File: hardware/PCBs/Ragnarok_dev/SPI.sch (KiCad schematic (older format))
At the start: 5 parts, among them U7 AB0815, U8 BMP388

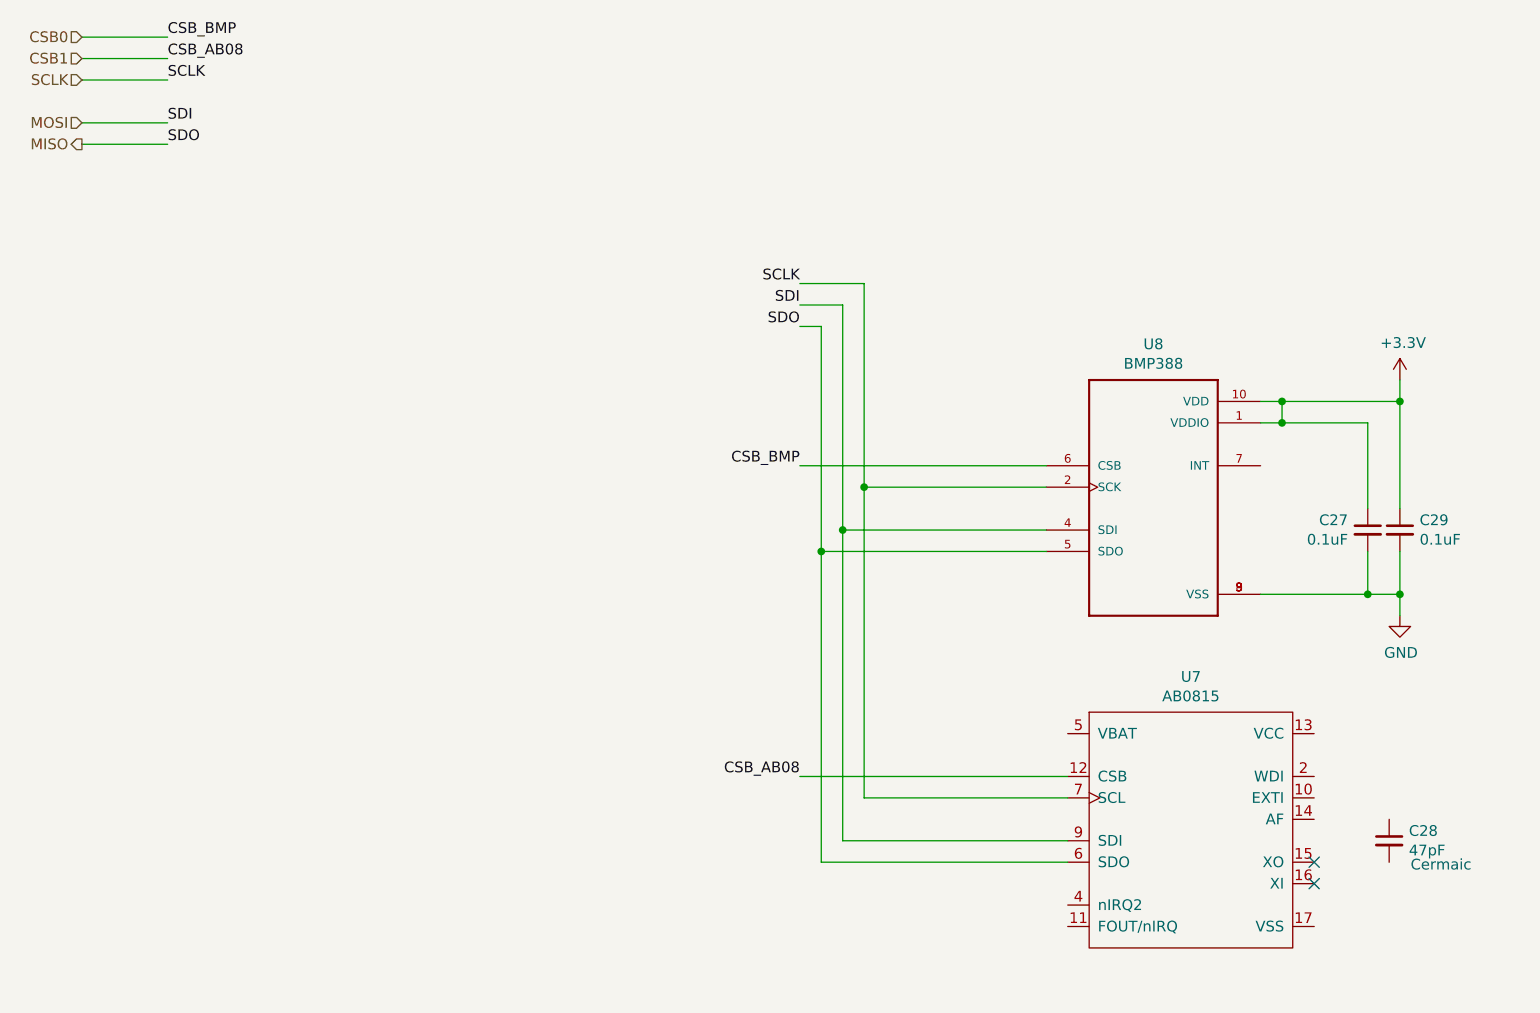
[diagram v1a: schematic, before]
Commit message: update
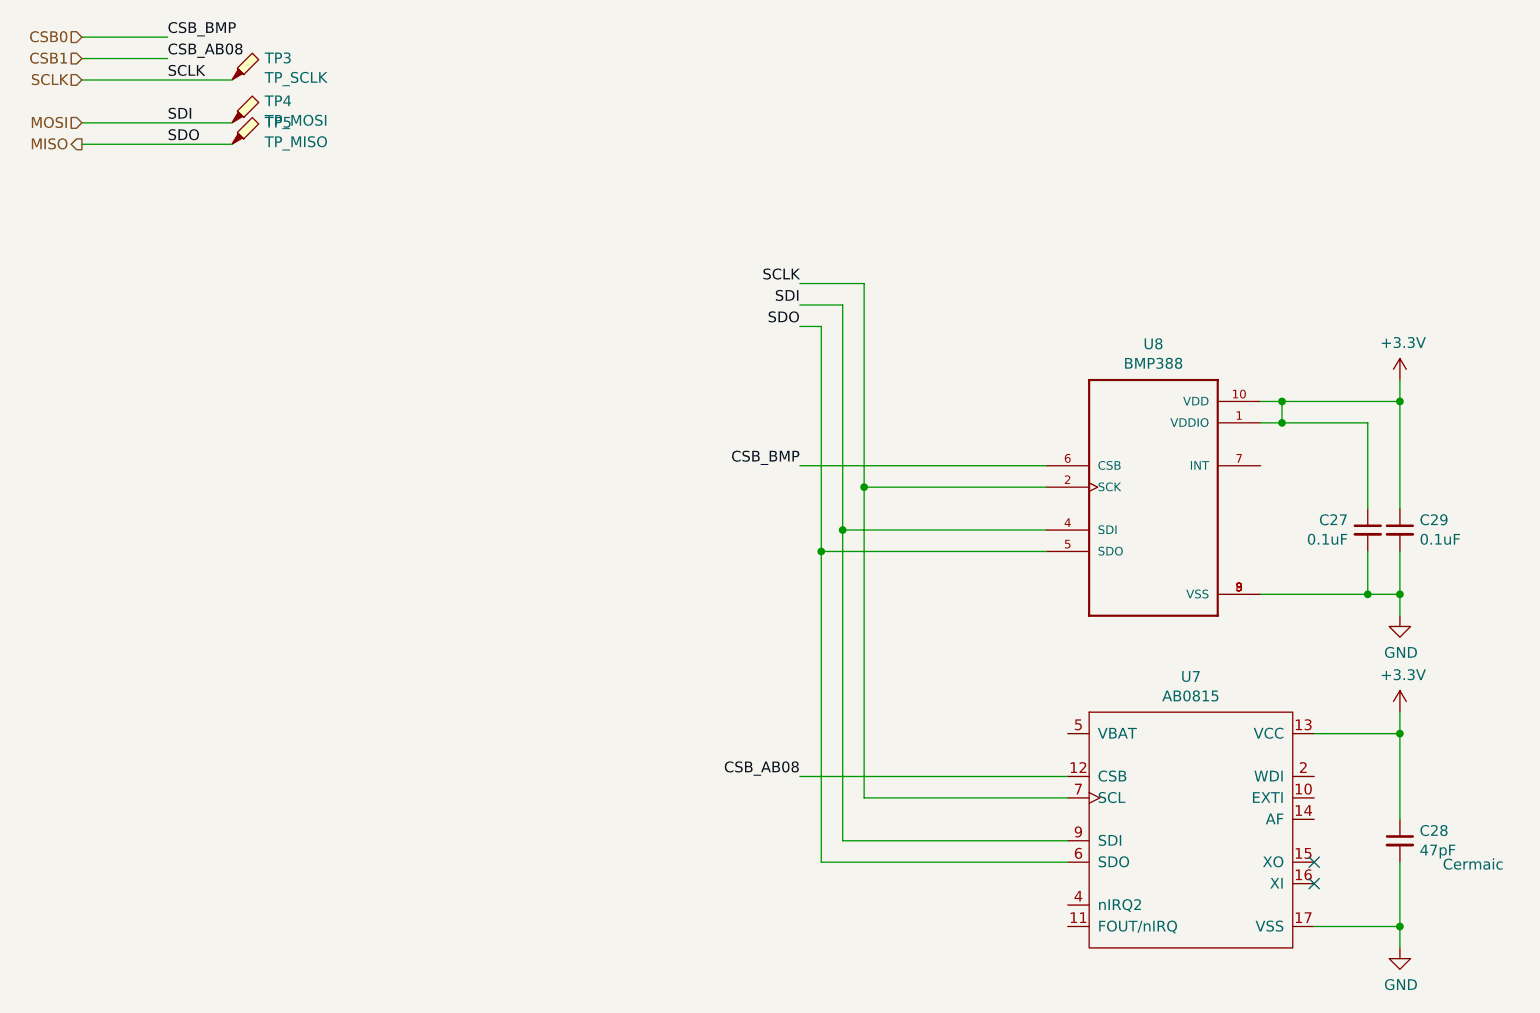
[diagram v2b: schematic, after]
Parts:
- added TP3: TP_SCLK, TestPoint:TestPoint_Pad_1.0x1.0mm, symbol Connector:TestPoint_Probe
- added TP4: TP_MOSI, TestPoint:TestPoint_Pad_1.0x1.0mm, symbol Connector:TestPoint_Probe
- added TP5: TP_MISO, TestPoint:TestPoint_Pad_1.0x1.0mm, symbol Connector:TestPoint_Probe
- C27, C28, C29: footprint (none) -> Capacitor_SMD:C_0603_1608Metric_Pad1.05x0.95mm_HandSolder
- U7: footprint (none) -> Package_DFN_QFN:QFN-16-1EP_5x5mm_P0.8mm_EP2.7x2.7mm
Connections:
- net +3V3: now also C28.1, U7.13 (VCC)
- net GND: now also C28.2, U7.17 (VSS)
- net MISO: now also TP5.1
- net MOSI: now also TP4.1
- net SCLK: now also TP3.1
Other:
- moved on the sheet: C28
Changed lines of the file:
@@
 F 0 "C29" H 7592 3446 50  0000 L CNN
 F 1 "0.1uF" H 7592 3355 50  0000 L CNN
-F 2 "" H 7500 3400 50  0001 C CNN
+F 2 "Capacitor_SMD:C_0603_1608Metric_Pad1.05x0.95mm_HandSolder" H 7500 3400 50  0001 C CNN
 F 3 "~" H 7500 3400 50  0001 C CNN
 	1    7500 3400
@@
 F 0 "U7" H 6525 4715 50  0000 C CNN
 F 1 "AB0815" H 6525 4624 50  0000 C CNN
-F 2 "" H 6550 4600 50  0001 C CNN
+F 2 "Package_DFN_QFN:QFN-16-1EP_5x5mm_P0.8mm_EP2.7x2.7mm" H 6550 4600 50  0001 C CNN
 F 3 "" H 6550 4600 50  0001 C CNN
 	1    5650 4400
@@
 L Device:C_Small C28
 U 1 1 5E1BCE97
-P 7450 4850
-F 0 "C28" H 7542 4896 50  0000 L CNN
-F 1 "47pF" H 7542 4805 50  0000 L CNN
-F 2 "" H 7450 4850 50  0001 C CNN
-F 3 "~" H 7450 4850 50  0001 C CNN
-	1    7450 4850
-	1    0    0    -1
-$EndComp
-Text Notes 7550 5000 0    50   ~ 0
+P 7500 4850
+F 0 "C28" H 7592 4896 50  0000 L CNN
+F 1 "47pF" H 7592 4805 50  0000 L CNN
+F 2 "Capacitor_SMD:C_0603_1608Metric_Pad1.05x0.95mm_HandSolder" H 7500 4850 50  0001 C CNN
+F 3 "~" H 7500 4850 50  0001 C CNN
+	1    7500 4850
+	1    0    0    -1
+$EndComp
+Text Notes 7700 5000 0    50   ~ 0
 Cermaic\n
 $Comp
@@
 F 0 "C27" H 7442 3446 50  0000 L CNN
 F 1 "0.1uF" H 7442 3355 50  0000 L CNN
-F 2 "" H 7350 3400 50  0001 C CNN
+F 2 "Capacitor_SMD:C_0603_1608Metric_Pad1.05x0.95mm_HandSolder" H 7350 3400 50  0001 C CNN
 F 3 "~" H 7350 3400 50  0001 C CNN
 	1    7350 3400
@@
 Text Label 1750 1600 0    50   ~ 0
 SDO
-Wire Wire Line
-	1350 1300 1750 1300
-Wire Wire Line
-	1350 1500 1750 1500
-Wire Wire Line
-	1350 1600 1750 1600
 Text HLabel 1350 1100 0    50   Input ~ 0
 CSB0
@@
 NoConn ~ 7100 4950
 NoConn ~ 7100 5050
+$Comp
+L Connector:TestPoint_Probe TP?
+U 1 1 5E857A15
+P 2050 1300
+AR Path="/5E857A15" Ref="TP?"  Part="1"
+AR Path="/5E1A0CB7/5E857A15" Ref="TP3"  Part="1"
+F 0 "TP3" H 2203 1401 50  0000 L CNN
+F 1 "TP_SCLK" H 2203 1310 50  0000 L CNN
+F 2 "TestPoint:TestPoint_Pad_1.0x1.0mm" H 2250 1300 50  0001 C CNN
+F 3 "~" H 2250 1300 50  0001 C CNN
+	1    2050 1300
+	1    0    0    -1
+$EndComp
+$Comp
+L Connector:TestPoint_Probe TP?
+U 1 1 5E857A1B
+P 2050 1600
+AR Path="/5E857A1B" Ref="TP?"  Part="1"
+AR Path="/5E1A0CB7/5E857A1B" Ref="TP5"  Part="1"
+F 0 "TP5" H 2203 1701 50  0000 L CNN
+F 1 "TP_MISO" H 2203 1610 50  0000 L CNN
+F 2 "TestPoint:TestPoint_Pad_1.0x1.0mm" H 2250 1600 50  0001 C CNN
+F 3 "~" H 2250 1600 50  0001 C CNN
+	1    2050 1600
+	1    0    0    -1
+$EndComp
+$Comp
+L Connector:TestPoint_Probe TP?
+U 1 1 5E857A21
+P 2050 1500
+AR Path="/5E857A21" Ref="TP?"  Part="1"
+AR Path="/5E1A0CB7/5E857A21" Ref="TP4"  Part="1"
+F 0 "TP4" H 2203 1601 50  0000 L CNN
+F 1 "TP_MOSI" H 2203 1510 50  0000 L CNN
+F 2 "TestPoint:TestPoint_Pad_1.0x1.0mm" H 2250 1500 50  0001 C CNN
+F 3 "~" H 2250 1500 50  0001 C CNN
+	1    2050 1500
+	1    0    0    -1
+$EndComp
+Wire Wire Line
+	1350 1500 2050 1500
+Wire Wire Line
+	1350 1600 2050 1600
+Wire Wire Line
+	1350 1300 2050 1300
+$Comp
+L power:+3.3V #PWR0165
+U 1 1 5E85DA72
+P 7500 4250
+F 0 "#PWR0165" H 7500 4100 50  0001 C CNN
+F 1 "+3.3V" H 7515 4423 50  0000 C CNN
+F 2 "" H 7500 4250 50  0001 C CNN
+F 3 "" H 7500 4250 50  0001 C CNN
+	1    7500 4250
+	1    0    0    -1
+$EndComp
+Wire Wire Line
+	7500 4250 7500 4350
+Wire Wire Line
+	7500 4350 7100 4350
+Wire Wire Line
+	7500 4350 7500 4750
+Connection ~ 7500 4350
+Wire Wire Line
+	7500 4950 7500 5250
+Wire Wire Line
+	7500 5250 7100 5250
+$Comp
+L power:GND #PWR0166
+U 1 1 5E8607AC
+P 7500 5350
+F 0 "#PWR0166" H 7500 5100 50  0001 C CNN
+F 1 "GND" H 7505 5177 50  0000 C CNN
+F 2 "" H 7500 5350 50  0001 C CNN
+F 3 "" H 7500 5350 50  0001 C CNN
+	1    7500 5350
+	1    0    0    -1
+$EndComp
+Wire Wire Line
+	7500 5250 7500 5350
+Connection ~ 7500 5250
 $EndSCHEMATC
